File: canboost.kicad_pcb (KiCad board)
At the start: 2 copper layers, 19 parts, among them IC1 MCP2551-I/SN, P1 CONN_10X2, P2 CONN_10X2, P3 CONN_2

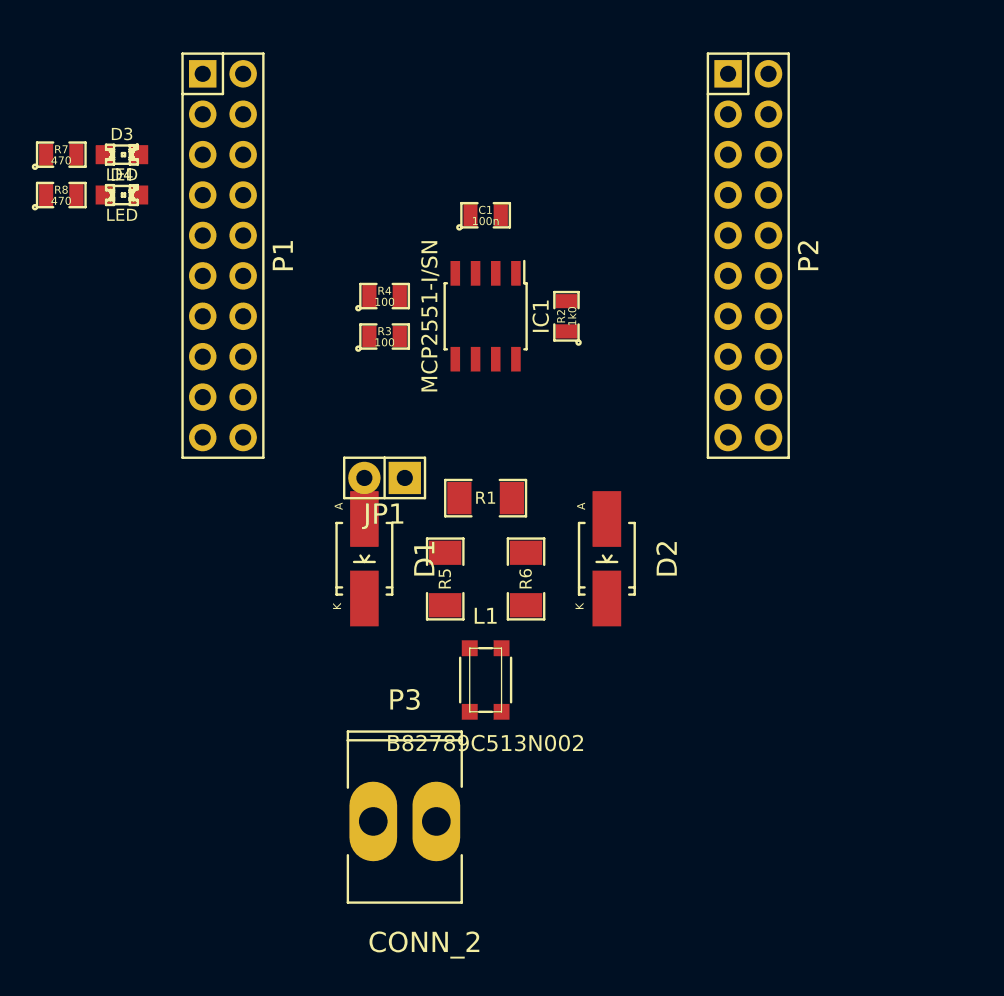
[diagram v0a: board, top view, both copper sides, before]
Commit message: layout complete (v0.10)
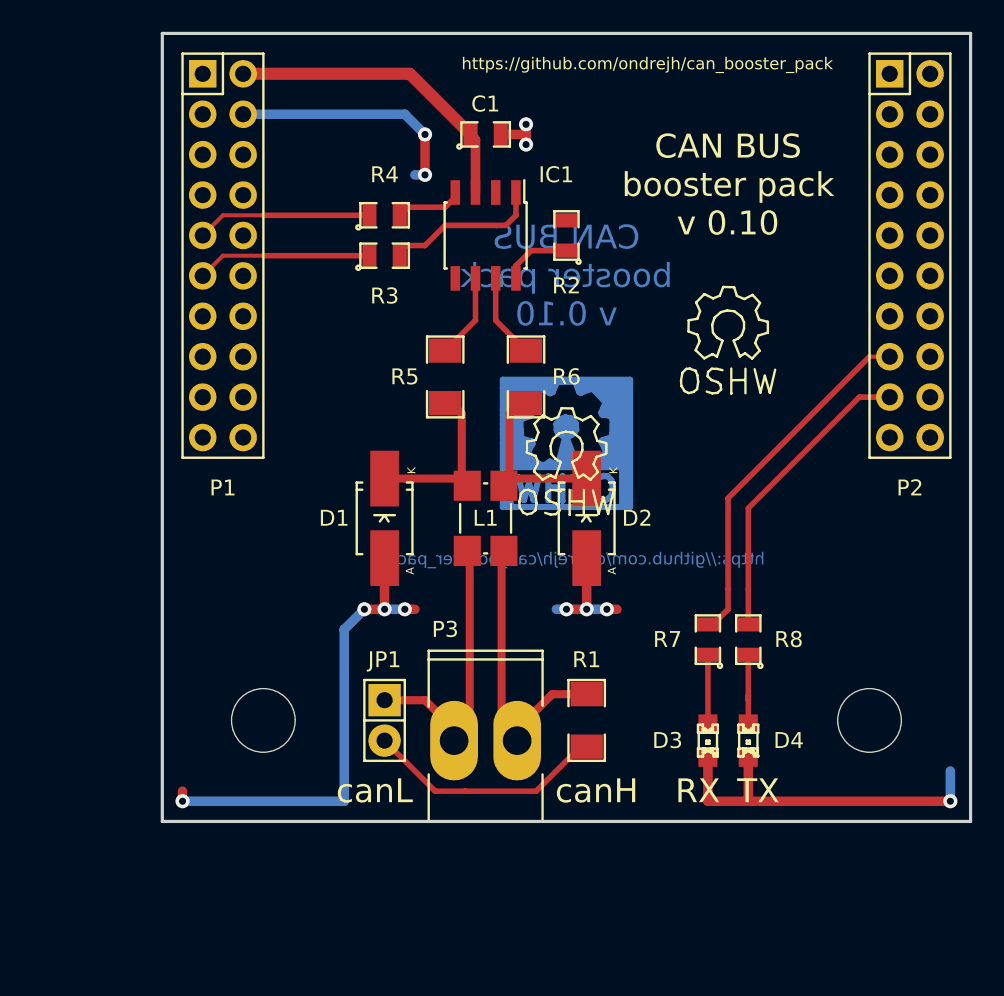
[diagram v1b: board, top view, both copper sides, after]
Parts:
- added MH: MountingHole_4mm_RevA_Date21Jun2010, Mounting_Holes:MountingHole_4mm, F.Cu at (99.1, 83.8)
- added MH: MountingHole_4mm_RevA_Date21Jun2010, Mounting_Holes:MountingHole_4mm, F.Cu at (61.0, 83.8)
- added SYM: Symbol_OSHW-Logo_CopperTop_Negative_07Jul2012, Symbols:Symbol_OSHW-Logo_CopperTop_Negative, B.Cu at (80.0, 65.4)
- added SYM: Symbol_OSHW-Logo_SilkScreen_07Jul2012, Symbols:Symbol_OSHW-Logo_SilkScreen, F.Cu at (90.2, 59.1)
- added SYM: Symbol_OSHW-Logo_SilkScreen_07Jul2012, Symbols:Symbol_OSHW-Logo_SilkScreen, F.Cu at (80.0, 66.7)
- moved D4 52.2 mm to (91.4, 85.1), turned to 270 degrees
- moved D3 52.1 mm to (88.9, 85.1), turned to 270 degrees
- moved R8 51.4 mm to (91.4, 78.7), turned to 90 degrees
- moved R7 50.8 mm to (88.9, 78.7), turned to 90 degrees
- moved R1 15.3 mm to (81.3, 83.8), turned to 90 degrees
- moved JP1 15.2 mm to (68.6, 83.8), turned to 270 degrees
- moved R5 12.7 mm to (72.4, 62.2)
- moved R6 12.7 mm to (77.5, 62.2)
- moved L1 10.2 mm to (74.9, 71.1)
- moved P2 10.2 mm to (101.6, 54.6)
- moved P3 7.18 mm to (74.9, 85.1)
- moved C1 5.08 mm to (74.9, 47.0)
- moved IC1 5.08 mm to (74.9, 53.3)
- moved R2 5.08 mm to (80.0, 53.3)
- moved R3 5.08 mm to (68.6, 54.6)
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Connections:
- D3 pad 2: PB0_LED_RX -> GND
- D4 pad 2: PB1_LED_TX -> GND
- IC1 pad 5: Net-(IC1-Pad5) -> (no net)
- JP1 pad 1: Net-(IC1-Pad6) -> CANL
- L1 pad 1: (no net) -> Net-(D1-Pad2)
- L1 pad 2: (no net) -> CANL
- L1 pad 3: (no net) -> CANH
- L1 pad 4: (no net) -> Net-(D2-Pad2)
- P1 pad 1: Net-(P1-Pad1) -> (no net)
- P1 pad 10: Net-(P1-Pad10) -> (no net)
- P1 pad 12: Net-(P1-Pad12) -> (no net)
- P1 pad 13: Net-(P1-Pad13) -> (no net)
- P1 pad 14: Net-(P1-Pad14) -> (no net)
- P1 pad 15: Net-(P1-Pad15) -> (no net)
- P1 pad 16: Net-(P1-Pad16) -> (no net)
- P1 pad 17: Net-(P1-Pad17) -> (no net)
- P1 pad 18: Net-(P1-Pad18) -> (no net)
- P1 pad 19: Net-(P1-Pad19) -> (no net)
- P1 pad 20: Net-(P1-Pad20) -> (no net)
- P1 pad 3: Net-(P1-Pad3) -> (no net)
- P1 pad 5: PB0_LED_RX -> (no net)
- P1 pad 6: Net-(P1-Pad6) -> (no net)
- P1 pad 7: PB1_LED_TX -> (no net)
- P1 pad 8: Net-(P1-Pad8) -> (no net)
- P2 pad 1: Net-(P2-Pad1) -> (no net)
- P2 pad 10: Net-(P2-Pad10) -> (no net)
- P2 pad 11: Net-(P2-Pad11) -> (no net)
- P2 pad 12: Net-(P2-Pad12) -> (no net)
- P2 pad 13: Net-(P2-Pad13) -> (no net)
- P2 pad 14: Net-(P2-Pad14) -> (no net)
- P2 pad 15: Net-(P2-Pad15) -> PB0_LED_RX
- P2 pad 16: Net-(P2-Pad16) -> (no net)
- P2 pad 17: Net-(P2-Pad17) -> PB1_LED_TX
- P2 pad 18: Net-(P2-Pad18) -> (no net)
- P2 pad 19: Net-(P2-Pad19) -> (no net)
- P2 pad 2: Net-(P2-Pad2) -> GND
- P2 pad 20: Net-(P2-Pad20) -> (no net)
- P2 pad 3: Net-(P2-Pad3) -> (no net)
- P2 pad 4: Net-(P2-Pad4) -> (no net)
- P2 pad 5: Net-(P2-Pad5) -> (no net)
- P2 pad 6: Net-(P2-Pad6) -> (no net)
- P2 pad 7: Net-(P2-Pad7) -> (no net)
- P2 pad 8: Net-(P2-Pad8) -> (no net)
- P2 pad 9: Net-(P2-Pad9) -> (no net)
- P3 pad 1: Net-(L1-Pad~) -> CANL
- P3 pad 2: Net-(L1-Pad~) -> CANH
- R1 pad 2: Net-(IC1-Pad7) -> CANH
- R7 pad 1: VDD -> Net-(D3-Pad1)
- R7 pad 2: Net-(D3-Pad1) -> PB0_LED_RX
- R8 pad 1: VDD -> Net-(D4-Pad1)
- R8 pad 2: Net-(D4-Pad1) -> PB1_LED_TX
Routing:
- net GND: track 0.00 -> 78.7 mm, vias 0 -> 12
- net PB0_LED_RX: track 0.00 -> 22.5 mm
- net VDD: track 0.00 -> 19.6 mm
- net PB1_LED_TX: track 0.00 -> 19.1 mm
- net CANH: track 0.00 -> 18.4 mm
- net CANL: track 0.00 -> 18.2 mm
- net Net-(JP1-Pad2): track 0.00 -> 15.2 mm
- net Net-(D1-Pad2): track 0.00 -> 11.7 mm
- net Net-(D2-Pad2): track 0.00 -> 11.7 mm
- net PE5_CAN0TX: track 0.00 -> 11.0 mm
- net PE4_CAN0RX: track 0.00 -> 11.0 mm
- net Net-(IC1-Pad1): track 0.00 -> 9.91 mm
- net Net-(IC1-Pad7): track 0.00 -> 5.33 mm
- net Net-(IC1-Pad6): track 0.00 -> 5.33 mm
- net Net-(D4-Pad1): track 0.00 -> 4.67 mm
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- added copper zone on B.Cu, net GND
- added copper zone on F.Cu, net GND
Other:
- board outline added: 50.8 x 49.5 mm
- net class BoardIO added: clearance 0.254, trace_width 0.5, via_dia 0.889, via_drill 0.635
- net class Default: trace_width 0.254 -> 0.35
- net class PWR added: clearance 0.254, trace_width 0.6, via_dia 0.889, via_drill 0.635
- board text added: "CAN BUS booster pack v 0.10"
- board text added: "RX"
- board text added: "TX"
- board text added: "canH"
- board text added: "canL"
- board text added: "https://github.com/ondrejh/can_booster_pack"
